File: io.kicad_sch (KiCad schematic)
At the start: 1 part, among them U201 xc7z010clg400

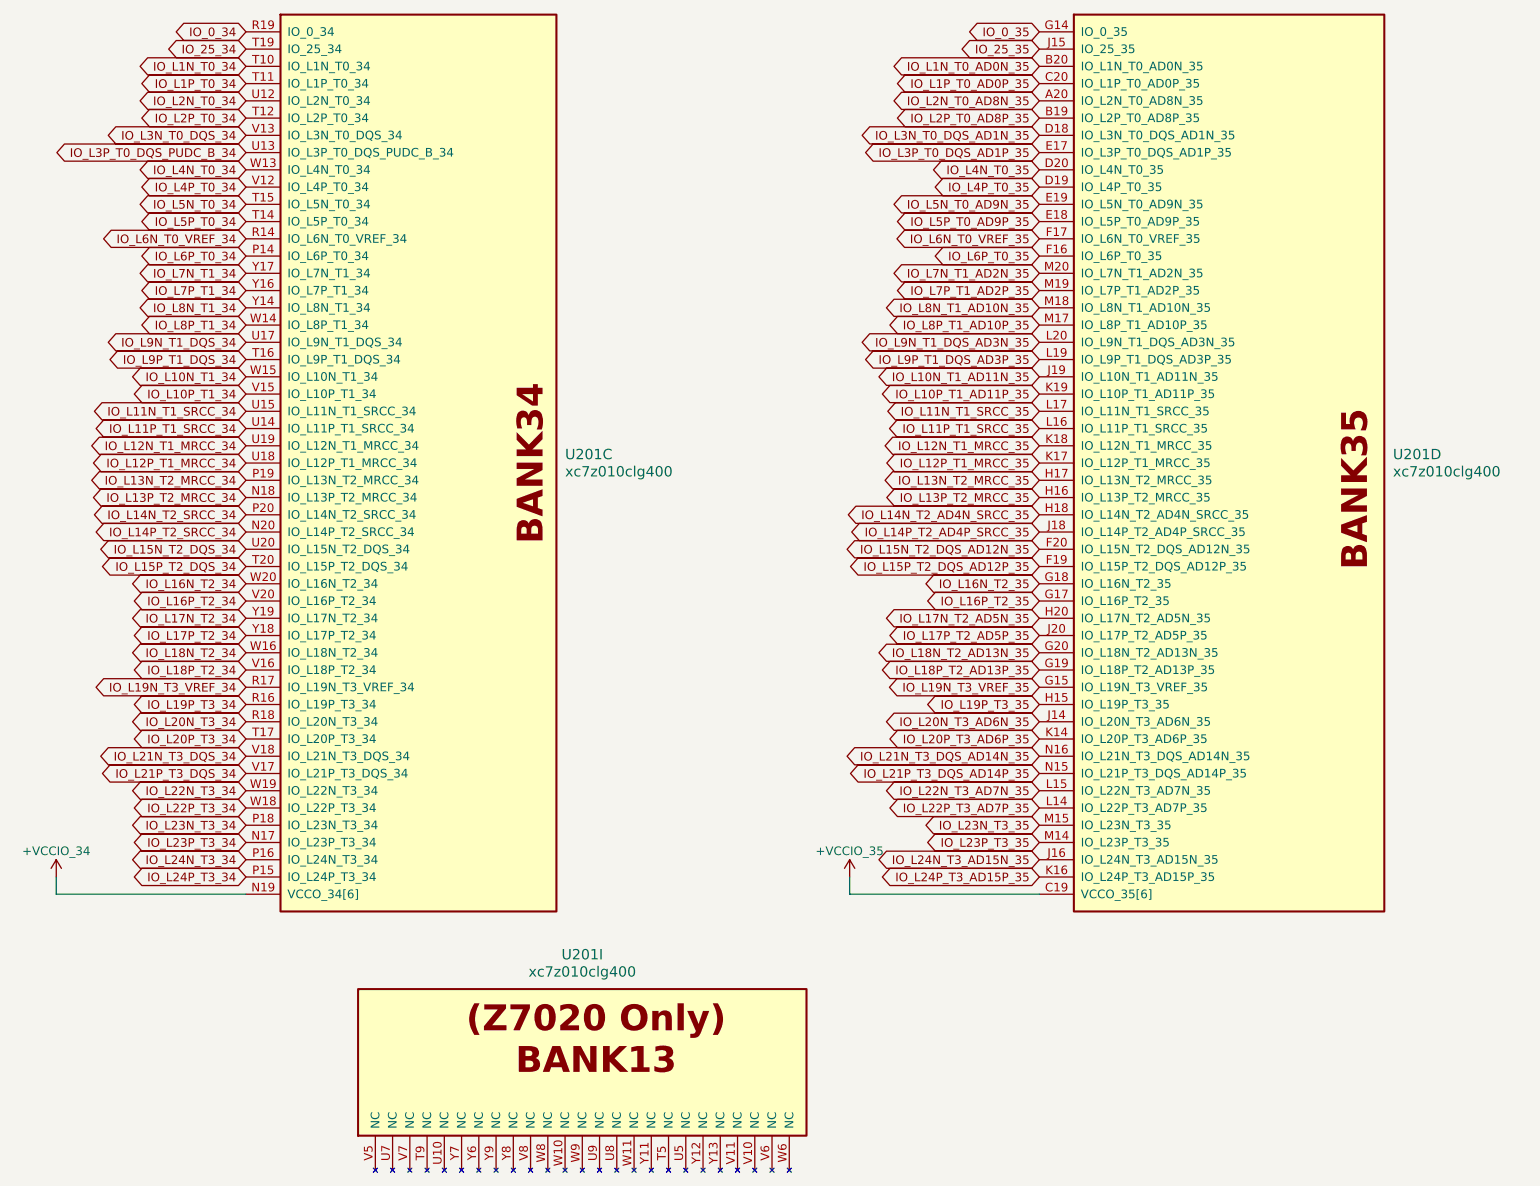
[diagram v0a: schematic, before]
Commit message: feat: continue improve sch design
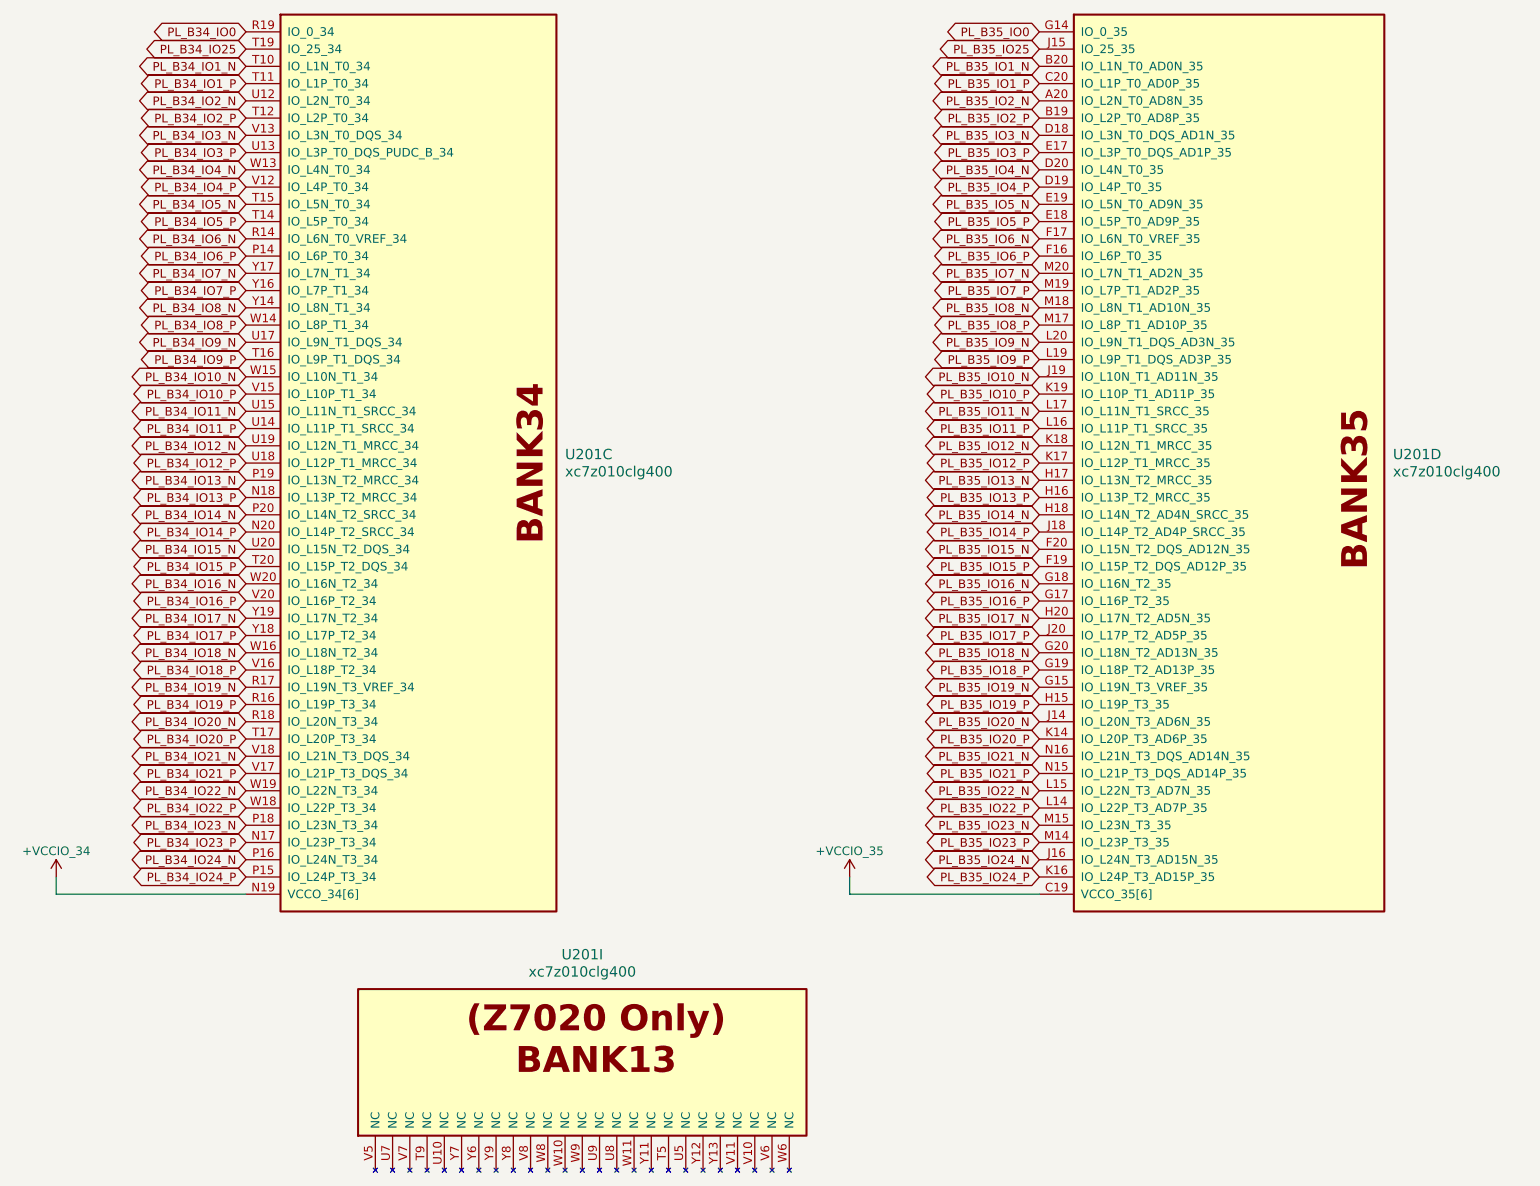
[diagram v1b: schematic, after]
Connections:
- net IO_0_34 renamed PL_B34_IO0
- net IO_0_35 renamed PL_B35_IO0
- net IO_25_34 renamed PL_B34_IO25
- net IO_25_35 renamed PL_B35_IO25
- net IO_L10N_T1_34 renamed PL_B34_IO10_N
- net IO_L10N_T1_AD11N_35 renamed PL_B35_IO10_N
- net IO_L10P_T1_34 renamed PL_B34_IO10_P
- net IO_L10P_T1_AD11P_35 renamed PL_B35_IO10_P
- net IO_L11N_T1_SRCC_34 renamed PL_B34_IO11_N
- net IO_L11N_T1_SRCC_35 renamed PL_B35_IO11_N
- net IO_L11P_T1_SRCC_34 renamed PL_B34_IO11_P
- net IO_L11P_T1_SRCC_35 renamed PL_B35_IO11_P
- net IO_L12N_T1_MRCC_34 renamed PL_B34_IO12_N
- net IO_L12N_T1_MRCC_35 renamed PL_B35_IO12_N
- net IO_L12P_T1_MRCC_34 renamed PL_B34_IO12_P
- net IO_L12P_T1_MRCC_35 renamed PL_B35_IO12_P
- net IO_L13N_T2_MRCC_34 renamed PL_B34_IO13_N
- net IO_L13N_T2_MRCC_35 renamed PL_B35_IO13_N
- net IO_L13P_T2_MRCC_34 renamed PL_B34_IO13_P
- net IO_L13P_T2_MRCC_35 renamed PL_B35_IO13_P
- net IO_L14N_T2_AD4N_SRCC_35 renamed PL_B35_IO14_N
- net IO_L14N_T2_SRCC_34 renamed PL_B34_IO14_N
- net IO_L14P_T2_AD4P_SRCC_35 renamed PL_B35_IO14_P
- net IO_L14P_T2_SRCC_34 renamed PL_B34_IO14_P
- net IO_L15N_T2_DQS_34 renamed PL_B34_IO15_N
- net IO_L15N_T2_DQS_AD12N_35 renamed PL_B35_IO15_N
- net IO_L15P_T2_DQS_34 renamed PL_B34_IO15_P
- net IO_L15P_T2_DQS_AD12P_35 renamed PL_B35_IO15_P
- net IO_L16N_T2_34 renamed PL_B34_IO16_N
- net IO_L16N_T2_35 renamed PL_B35_IO16_N
- net IO_L16P_T2_34 renamed PL_B34_IO16_P
- net IO_L16P_T2_35 renamed PL_B35_IO16_P
- net IO_L17N_T2_34 renamed PL_B34_IO17_N
- net IO_L17N_T2_AD5N_35 renamed PL_B35_IO17_N
- net IO_L17P_T2_34 renamed PL_B34_IO17_P
- net IO_L17P_T2_AD5P_35 renamed PL_B35_IO17_P
- net IO_L18N_T2_34 renamed PL_B34_IO18_N
- net IO_L18N_T2_AD13N_35 renamed PL_B35_IO18_N
- net IO_L18P_T2_34 renamed PL_B34_IO18_P
- net IO_L18P_T2_AD13P_35 renamed PL_B35_IO18_P
- net IO_L19N_T3_VREF_34 renamed PL_B34_IO19_N
- net IO_L19N_T3_VREF_35 renamed PL_B35_IO19_N
- net IO_L19P_T3_34 renamed PL_B34_IO19_P
- net IO_L19P_T3_35 renamed PL_B35_IO19_P
- net IO_L1N_T0_34 renamed PL_B34_IO1_N
- net IO_L1N_T0_AD0N_35 renamed PL_B35_IO1_N
- net IO_L1P_T0_34 renamed PL_B34_IO1_P
- net IO_L1P_T0_AD0P_35 renamed PL_B35_IO1_P
- net IO_L20N_T3_34 renamed PL_B34_IO20_N
- net IO_L20N_T3_AD6N_35 renamed PL_B35_IO20_N
- net IO_L20P_T3_34 renamed PL_B34_IO20_P
- net IO_L20P_T3_AD6P_35 renamed PL_B35_IO20_P
- net IO_L21N_T3_DQS_34 renamed PL_B34_IO21_N
- net IO_L21N_T3_DQS_AD14N_35 renamed PL_B35_IO21_N
- net IO_L21P_T3_DQS_34 renamed PL_B34_IO21_P
- net IO_L21P_T3_DQS_AD14P_35 renamed PL_B35_IO21_P
- net IO_L22N_T3_34 renamed PL_B34_IO22_N
- net IO_L22N_T3_AD7N_35 renamed PL_B35_IO22_N
- net IO_L22P_T3_34 renamed PL_B34_IO22_P
- net IO_L22P_T3_AD7P_35 renamed PL_B35_IO22_P
- net IO_L23N_T3_34 renamed PL_B34_IO23_N
- net IO_L23N_T3_35 renamed PL_B35_IO23_N
- net IO_L23P_T3_34 renamed PL_B34_IO23_P
- net IO_L23P_T3_35 renamed PL_B35_IO23_P
- net IO_L24N_T3_34 renamed PL_B34_IO24_N
- net IO_L24N_T3_AD15N_35 renamed PL_B35_IO24_N
- net IO_L24P_T3_34 renamed PL_B34_IO24_P
- net IO_L24P_T3_AD15P_35 renamed PL_B35_IO24_P
- net IO_L2N_T0_34 renamed PL_B34_IO2_N
- net IO_L2N_T0_AD8N_35 renamed PL_B35_IO2_N
- net IO_L2P_T0_34 renamed PL_B34_IO2_P
- net IO_L2P_T0_AD8P_35 renamed PL_B35_IO2_P
- net IO_L3N_T0_DQS_34 renamed PL_B34_IO3_N
- net IO_L3N_T0_DQS_AD1N_35 renamed PL_B35_IO3_N
- net IO_L3P_T0_DQS_AD1P_35 renamed PL_B35_IO3_P
- net IO_L3P_T0_DQS_PUDC_B_34 renamed PL_B34_IO3_P
- net IO_L4N_T0_34 renamed PL_B34_IO4_N
- net IO_L4N_T0_35 renamed PL_B35_IO4_N
- net IO_L4P_T0_34 renamed PL_B34_IO4_P
- net IO_L4P_T0_35 renamed PL_B35_IO4_P
- net IO_L5N_T0_34 renamed PL_B34_IO5_N
- net IO_L5N_T0_AD9N_35 renamed PL_B35_IO5_N
- net IO_L5P_T0_34 renamed PL_B34_IO5_P
- net IO_L5P_T0_AD9P_35 renamed PL_B35_IO5_P
- net IO_L6N_T0_VREF_34 renamed PL_B34_IO6_N
- net IO_L6N_T0_VREF_35 renamed PL_B35_IO6_N
- net IO_L6P_T0_34 renamed PL_B34_IO6_P
- net IO_L6P_T0_35 renamed PL_B35_IO6_P
- net IO_L7N_T1_34 renamed PL_B34_IO7_N
- net IO_L7N_T1_AD2N_35 renamed PL_B35_IO7_N
- net IO_L7P_T1_34 renamed PL_B34_IO7_P
- net IO_L7P_T1_AD2P_35 renamed PL_B35_IO7_P
- net IO_L8N_T1_34 renamed PL_B34_IO8_N
- net IO_L8N_T1_AD10N_35 renamed PL_B35_IO8_N
- net IO_L8P_T1_34 renamed PL_B34_IO8_P
- net IO_L8P_T1_AD10P_35 renamed PL_B35_IO8_P
- net IO_L9N_T1_DQS_34 renamed PL_B34_IO9_N
- net IO_L9N_T1_DQS_AD3N_35 renamed PL_B35_IO9_N
- net IO_L9P_T1_DQS_34 renamed PL_B34_IO9_P
- net IO_L9P_T1_DQS_AD3P_35 renamed PL_B35_IO9_P
